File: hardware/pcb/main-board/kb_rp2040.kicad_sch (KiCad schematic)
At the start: 28 parts, among them J1201 Conn_01x02, J1202 Conn_01x02, U1202 W25Q32JVSNIQ, U1203 RP2040, Y1201 ABLS-12.000MHZ-B4-T

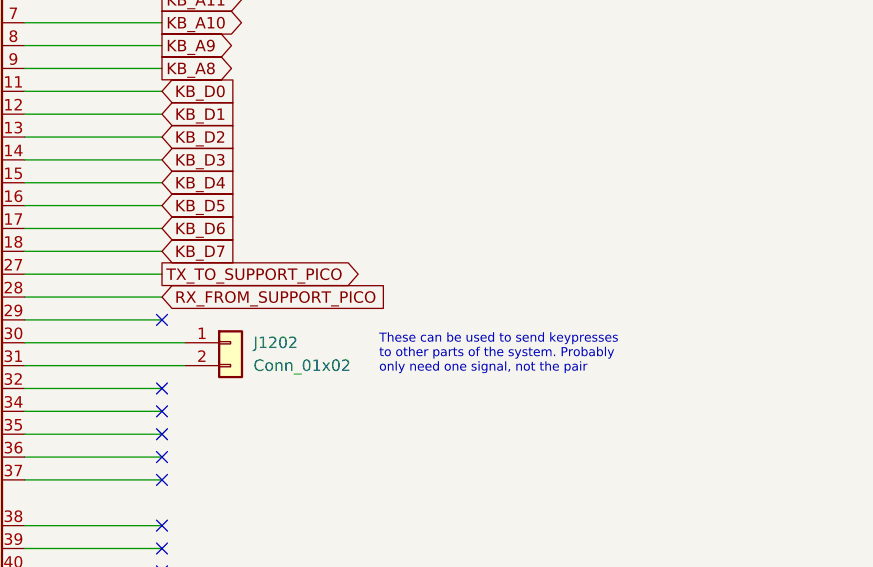
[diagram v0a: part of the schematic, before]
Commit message: more support rp2040 cleanups
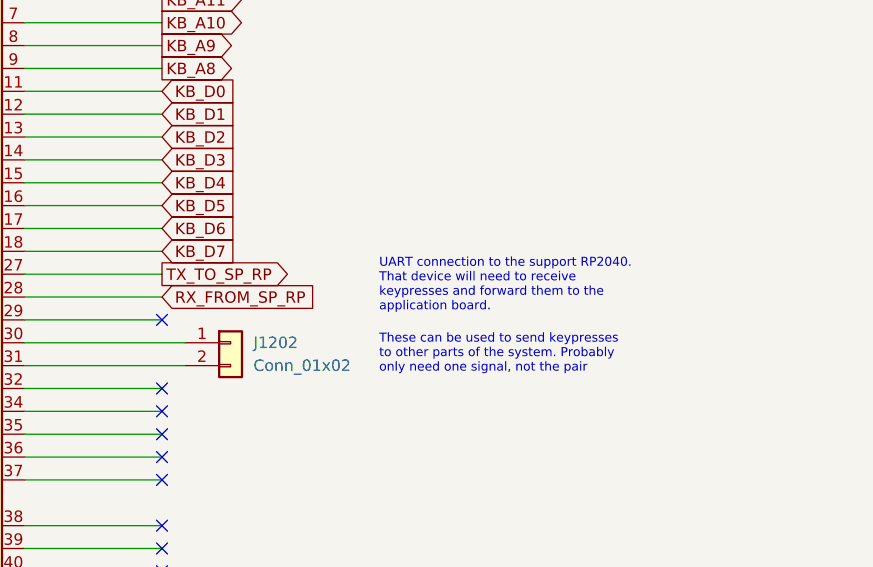
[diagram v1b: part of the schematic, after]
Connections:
- net RX_FROM_SUPPORT_PICO renamed RX_FROM_SP_RP
- net TX_TO_SUPPORT_PICO renamed TX_TO_SP_RP
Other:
- note added: "UART connection to the support RP2040. That device will need to receive keypresses and forward them to the application board."
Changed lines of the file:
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@@
+		)
+	)
+	(text "UART connection to the support RP2040.\nThat device will need to receive\nkeypresses and forward them to the\napplication board."
+		(exclude_from_sim no)
+		(at 144.78 119.38 0)
+		(effects
+			(font
+				(size 1 1)
+			)
+			(justify left)
 		)
 	)
@@
 		)
 	)
-	(global_label "TX_TO_SUPPORT_PICO"
+	(global_label "TX_TO_SP_RP"
 		(shape output)
 		(at 120.65 118.11 0)
@@
 		)
 		(property "Intersheetrefs" "${INTERSHEET_REFS}"
-			(at 143.4824 118.11 0)
+			(at 135.3785 118.11 0)
 			(effects
 				(font
@@
 		)
 	)
-	(global_label "RX_FROM_SUPPORT_PICO"
+	(global_label "RX_FROM_SP_RP"
 		(shape input)
 		(at 120.65 120.65 0)
@@
 		)
 		(property "Intersheetrefs" "${INTERSHEET_REFS}"
-			(at 146.6272 120.65 0)
-			(effects
-				(font
+			(at 138.5233 120.65 0)
+			(effects
+				(font

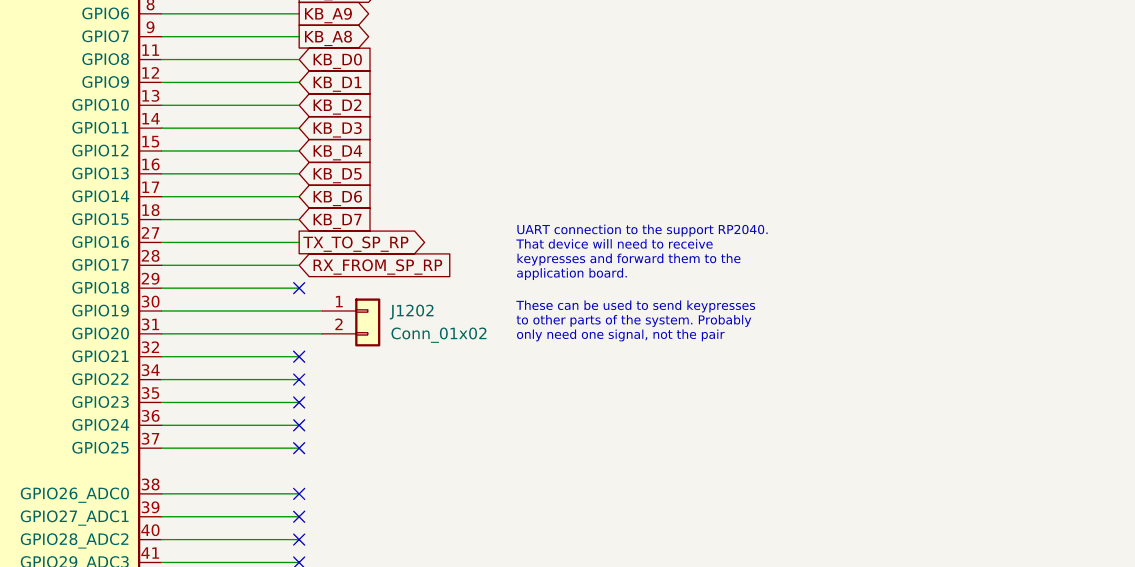
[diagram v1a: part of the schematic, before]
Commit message: tidy the keyboard comms
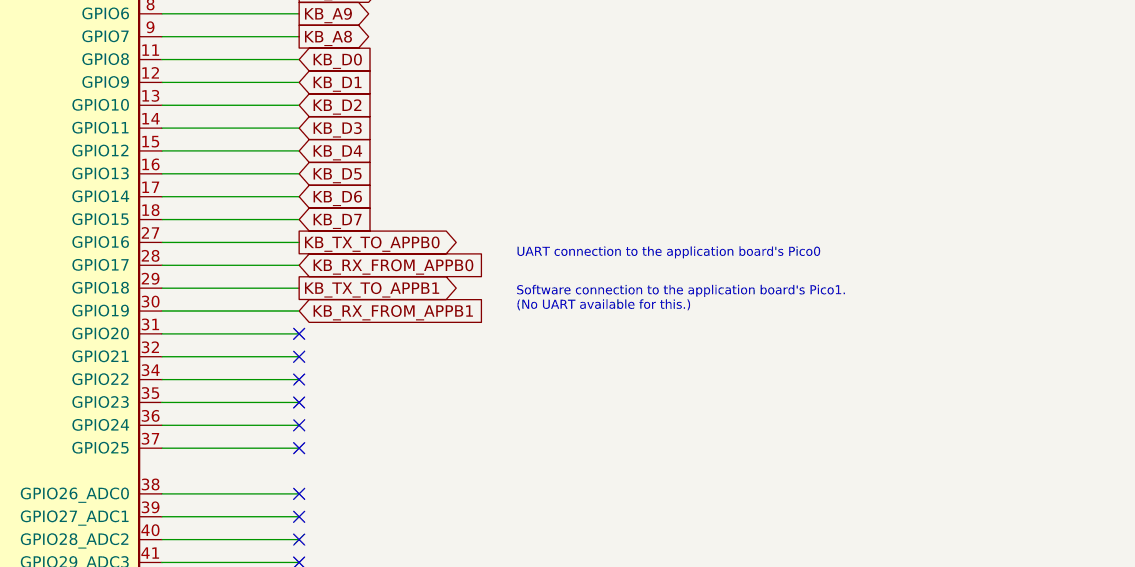
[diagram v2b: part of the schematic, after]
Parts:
- removed J1202: Conn_01x02, symbol Connector_Generic:Conn_01x02
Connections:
- net KB_TX_TO_APPB1: now reaches U1203.29 (GPIO18)
- net KB_RX_FROM_APPB1: now reaches U1203.30 (GPIO19)
- net RX_FROM_SP_RP renamed KB_RX_FROM_APPB0
- net TX_TO_SP_RP renamed KB_TX_TO_APPB0
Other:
- note added: "Software connection to the application board's Pico1. (No UART available for this.)"
- note added: "UART connection to the application board's Pico0"
- note removed: "These can be used to send keypresses to other parts of the system. Probably only need one signal, not the pair"
- note removed: "UART connection to the support RP2040. That device will need to receive keypresses and forward them to the application board."
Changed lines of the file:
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@@
 	)
 	(no_connect
-		(at 120.65 130.81)
+		(at 120.65 128.27)
 	)
 	(no_connect
-		(at 120.65 146.05)
+		(at 120.65 130.81)
 	)
 	(no_connect
-		(at 120.65 123.19)
+		(at 120.65 146.05)
 	)
 	(no_connect
@@
 	(wire
 		(pts
-			(xy 105.41 125.73) (xy 123.19 125.73)
+			(xy 105.41 125.73) (xy 120.65 125.73)
 		)
 		(stroke
@@
 	(wire
 		(pts
-			(xy 105.41 128.27) (xy 123.19 128.27)
+			(xy 105.41 128.27) (xy 120.65 128.27)
 		)
 		(stroke
@@
 		)
 	)
+	(text "Software connection to the application board's Pico1.\n(No UART available for this.)"
+		(exclude_from_sim no)
+		(at 144.78 124.46 0)
+		(effects
+			(font
+				(size 1 1)
+			)
+			(justify left)
+		)
+	)
 	(text "Enabled by RP2040. Don't bother with the\nBOOTSEL switch unless there's a problem."
 		(exclude_from_sim no)
@@
 		)
 	)
-	(text "UART connection to the support RP2040.\nThat device will need to receive\nkeypresses and forward them to the\napplication board."
+	(text "UART connection to the application board's Pico0"
 		(exclude_from_sim no)
 		(at 144.78 119.38 0)
@@
 		)
 	)
-	(text "These can be used to send keypresses\nto other parts of the system. Probably\nonly need one signal, not the pair"
-		(exclude_from_sim no)
-		(at 144.78 127 0)
-		(effects
-			(font
-				(size 1 1)
-			)
-			(justify left)
-		)
-	)
 	(label "XOUT"
 		(at 275.59 100.33 180)
@@
 		)
 	)
-	(global_label "TX_TO_SP_RP"
+	(global_label "KB_TX_TO_APPB0"
 		(shape output)
 		(at 120.65 118.11 0)
@@
 		)
 		(property "Intersheetrefs" "${INTERSHEET_REFS}"
-			(at 135.3785 118.11 0)
+			(at 139.0071 118.11 0)
 			(effects
 				(font
@@
 		)
 	)
+	(global_label "KB_TX_TO_APPB1"
+		(shape output)
+		(at 120.65 123.19 0)
+		(fields_autoplaced yes)
+		(effects
+			(font
+				(size 1.27 1.27)
+			)
+			(justify left)
+		)
+		(property "Intersheetrefs" "${INTERSHEET_REFS}"
+			(at 139.0071 123.19 0)
+			(effects
+				(font
+					(size 1.27 1.27)
+				)
+				(justify left)
+				(hide yes)
+			)
+		)
+	)
 	(global_label "KB_A10"
 		(shape output)
@@
 		)
 	)
-	(global_label "RX_FROM_SP_RP"
+	(global_label "KB_RX_FROM_APPB0"
 		(shape input)
 		(at 120.65 120.65 0)
@@
 		)
 		(property "Intersheetrefs" "${INTERSHEET_REFS}"
-			(at 138.5233 120.65 0)
+			(at 142.1519 120.65 0)
+			(effects
+				(font
+					(size 1.27 1.27)
+				)
+				(justify left)
+				(hide yes)
+			)
+		)
+	)
+	(global_label "KB_RX_FROM_APPB1"
+		(shape input)
+		(at 120.65 125.73 0)
+		(fields_autoplaced yes)
+		(effects
+			(font
+				(size 1.27 1.27)
+			)
+			(justify left)
+		)
+		(property "Intersheetrefs" "${INTERSHEET_REFS}"
+			(at 142.1519 125.73 0)
 			(effects
 				(font
@@
 					(unit 1)
 				)
-			)
-		)
-	)
-	(symbol
-		(lib_id "Connector_Generic:Conn_01x02")
-		(at 128.27 125.73 0)
-		(unit 1)
-		(exclude_from_sim no)
-		(in_bom yes)
-		(on_board yes)
-		(dnp no)
-		(fields_autoplaced yes)
-		(property "Reference" "J1202"
-			(at 130.81 125.7299 0)
-			(effects
-				(font
-					(size 1.27 1.27)
-				)
-				(justify left)
-			)
-		)
-		(property "Value" "Conn_01x02"
-			(at 130.81 128.2699 0)
-			(effects
-				(font
-					(size 1.27 1.27)
-				)
-				(justify left)
-			)
-		)
-		(property "Footprint" ""
-			(at 128.27 125.73 0)
-			(effects
-				(font
-					(size 1.27 1.27)
-				)
-				(hide yes)
-			)
-		)
-		(property "Datasheet" "~"
-			(at 128.27 125.73 0)
-			(effects
-				(font
-					(size 1.27 1.27)
-				)
-				(hide yes)
-			)
-		)
-		(property "Description" "Generic connector, single row, 01x02, script generated (kicad-library-utils/schlib/autogen/connector/)"
-			(at 128.27 125.73 0)
-			(effects
-				(font
-					(size 1.27 1.27)
-				)
-				(hide yes)
-			)
-		)
-		(pin "2"
-		)
-		(pin "1"
-		)
-		(instances
-			(project ""
-				(path "/fdce8012-5f35-4f58-8abb-80214b4af8fe/bd010eea-67e1-4f0f-9c21-5375d46a1c97"
-					(reference "J1202")
-					(unit 1)
-				)
